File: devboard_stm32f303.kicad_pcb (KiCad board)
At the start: 2 copper layers, 50 x 17.8 mm, 20 parts, among them J2 USB_B_Mini, J3 Conn_01x20, J4 Conn_01x20, U1 STM32F303CCTx, U2 AMS1117-3.3, Y1 Crystal_Small

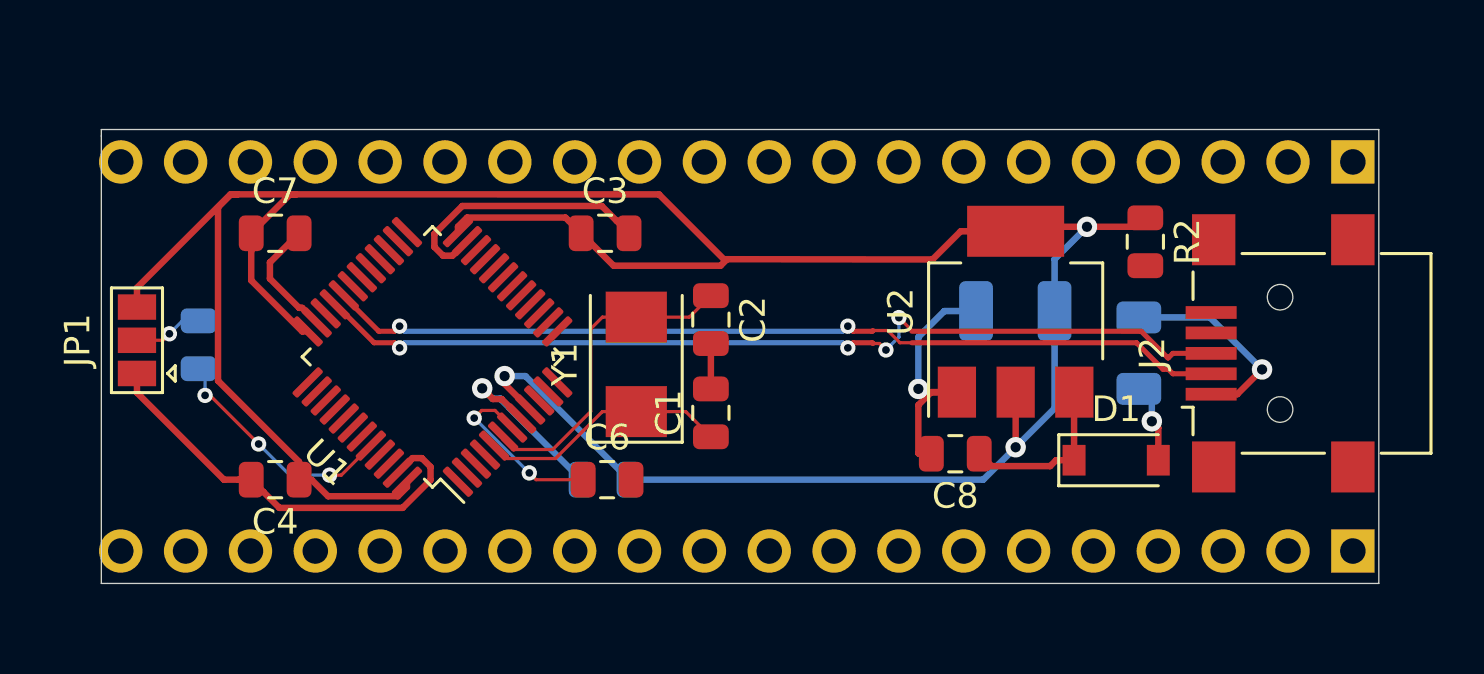
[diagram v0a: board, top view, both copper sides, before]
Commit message: New board layout
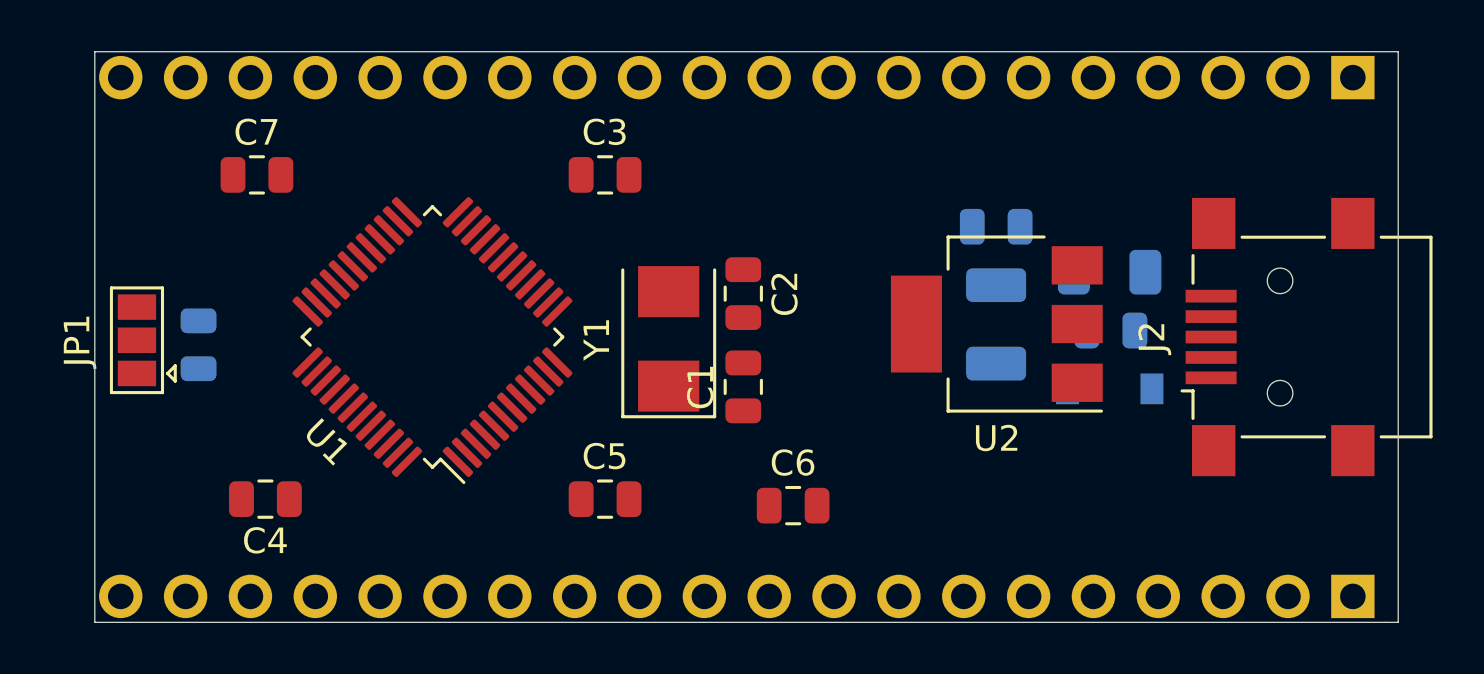
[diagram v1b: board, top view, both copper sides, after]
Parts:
- C5: moved to F.Cu
- C8, D1, R2: moved to B.Cu
- moved C8 9.03 mm to (126.7, 26.2)
- moved C6 7.36 mm to (118.8, 37.1)
- moved R2 3.73 mm to (131.2, 30.2), turned to 0 degrees
- moved F1 3.37 mm to (131.2, 27.9), turned to 180 degrees
- moved J3 3.30 mm to (140.7, 20.3)
- moved D1 2.81 mm to (131.2, 32.5)
- moved C7 2.39 mm to (97.8, 24.1)
- moved C3 2.29 mm to (111.4, 24.1)
- moved J4 1.78 mm to (140.7, 40.6)
- moved C2 1.63 mm to (116.8, 28.8)
- moved C1 1.63 mm to (116.8, 32.4)
- moved Y1 1.62 mm to (113.9, 30.6)
- moved C9 0.91 mm to (126.7, 30.0), turned to 270 degrees
- moved U2 0.88 mm to (126.8, 30.0), turned to 180 degrees
- moved C4 0.85 mm to (98.1, 36.8)
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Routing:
- net +3V3: track 117.0 -> 0.00 mm, vias 3 -> 0
- net GND: track 51.8 -> 0.00 mm, vias 2 -> 0
- net D+: track 37.1 -> 0.00 mm, vias 4 -> 0
- net D-: track 35.6 -> 0.00 mm, vias 2 -> 0
- net OSC_OUT: track 12.8 -> 0.00 mm
- net OSC_IN: track 9.87 -> 0.00 mm
- net BOOT0: track 9.60 -> 0.00 mm, vias 3 -> 0
- net Net-(F1-Pad1): track 8.07 -> 0.00 mm, vias 1 -> 0
- net RESET: track 7.16 -> 0.00 mm, vias 2 -> 0
- net Net-(C8-Pad1): track 6.68 -> 0.00 mm
- net VBUS: track 3.11 -> 0.00 mm, vias 1 -> 0
- net Net-(JP1-Pad2): track 2.73 -> 0.00 mm, vias 1 -> 0
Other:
- board size 50 x 17.8 mm -> 51.1 x 22.4 mm
- net class Default: clearance 0.2 -> 0.127
- net class Power: clearance 0.2 -> 0.1905
- rule trace_clearance: 0.2 -> 0.127
